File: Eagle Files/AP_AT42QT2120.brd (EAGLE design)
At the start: 36 x 45.6 mm, 20 parts

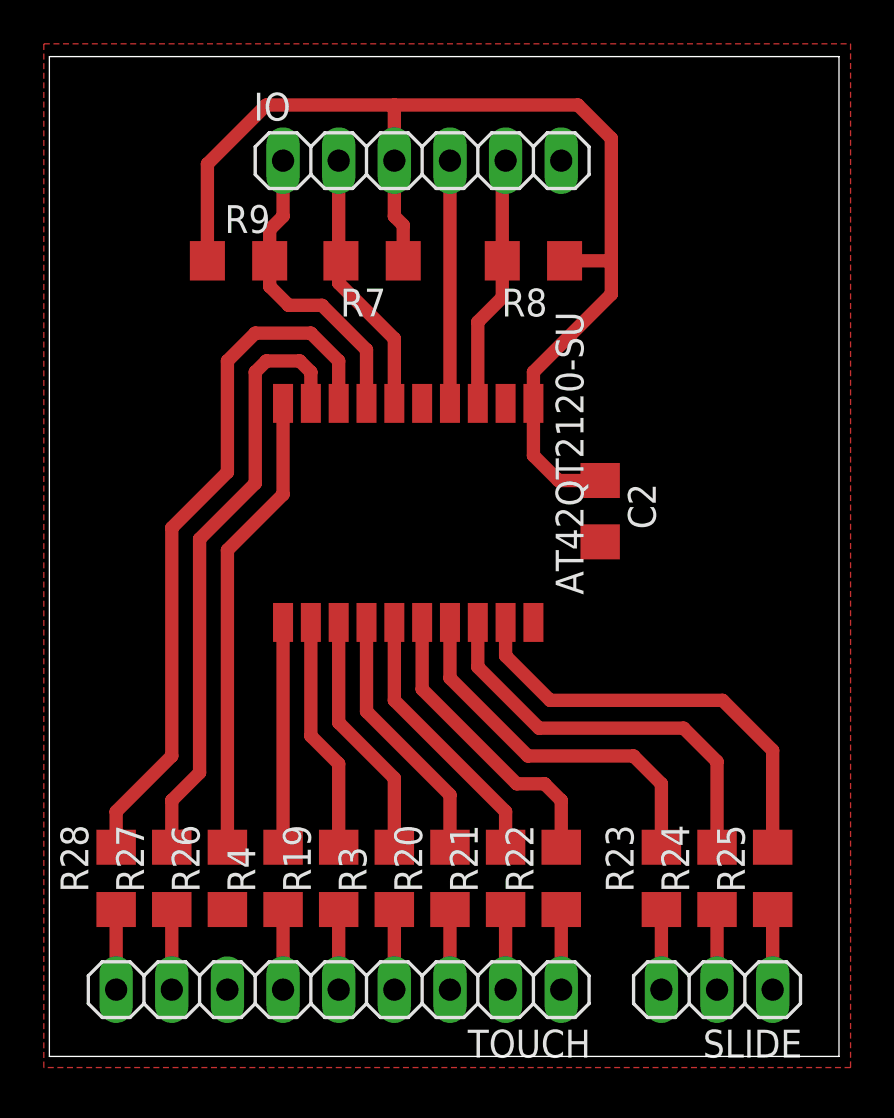
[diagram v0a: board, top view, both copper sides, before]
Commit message: pcb changes
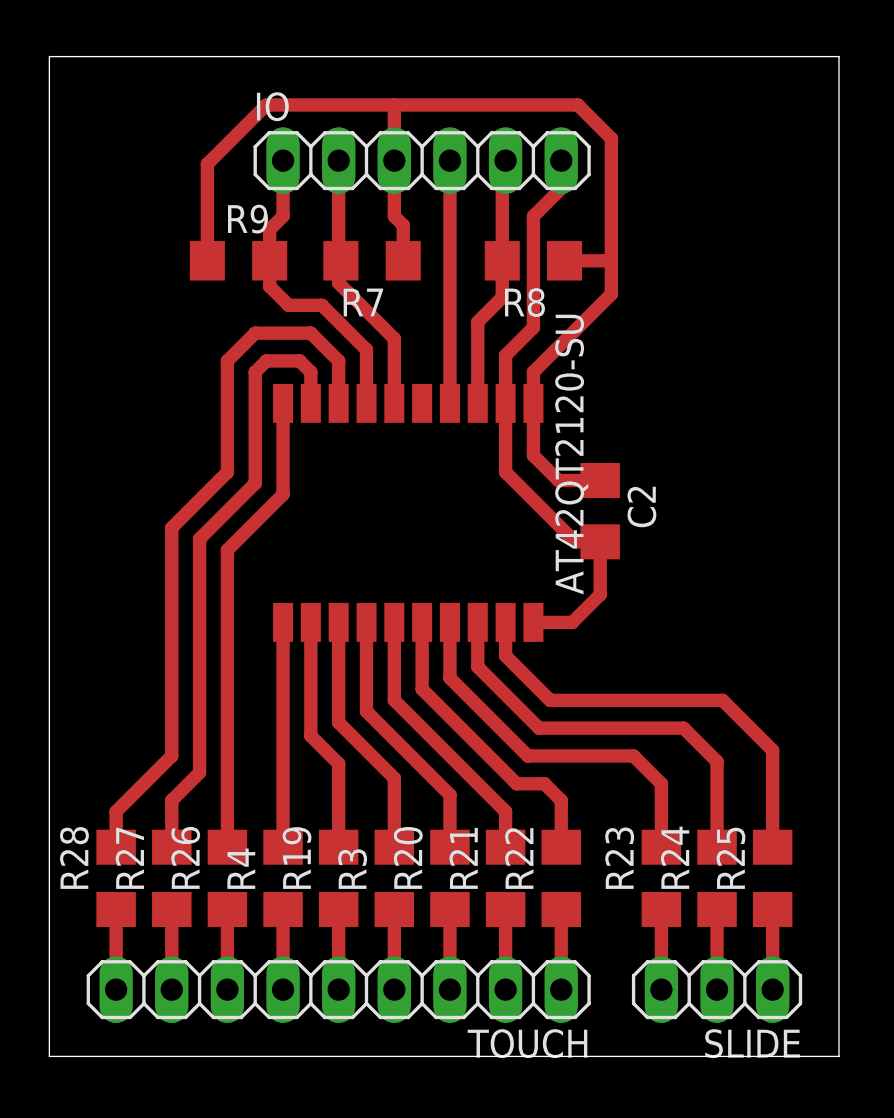
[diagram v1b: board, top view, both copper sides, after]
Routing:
- net GND: track 0.00 -> 26.9 mm
- net N$19: track 0.00 -> 3.66 mm
- removed copper zone on layer 1, net GND
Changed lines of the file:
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@@
 <contactref element="C2" pad="2"/>
 <contactref element="IO" pad="6"/>
-<polygon width="0.3048" layer="1">
-<vertex x="-0.254" y="-0.508"/>
-<vertex x="-0.254" y="46.228"/>
-<vertex x="36.576" y="46.228"/>
-<vertex x="36.576" y="-0.508"/>
-</polygon>
 <contactref element="U$1" pad="12"/>
 <contactref element="U$1" pad="10"/>
+<wire x1="23.368" y1="40.894" x2="23.368" y2="39.624" width="0.6096" layer="1"/>
+<wire x1="23.368" y1="39.624" x2="22.098" y2="38.354" width="0.6096" layer="1"/>
+<wire x1="22.098" y1="38.354" x2="22.098" y2="33.274" width="0.6096" layer="1"/>
+<wire x1="22.098" y1="33.274" x2="20.828" y2="32.004" width="0.6096" layer="1"/>
+<wire x1="20.828" y1="32.004" x2="20.828" y2="29.812" width="0.6096" layer="1"/>
+<wire x1="20.828" y1="29.812" x2="20.828" y2="26.67" width="0.6096" layer="1"/>
+<wire x1="24.006" y1="23.492" x2="25.146" y2="23.492" width="0.6096" layer="1"/>
+<wire x1="20.828" y1="26.67" x2="24.006" y2="23.492" width="0.6096" layer="1"/>
+<wire x1="22.098" y1="19.812" x2="23.876" y2="19.812" width="0.6096" layer="1"/>
+<wire x1="23.876" y1="19.812" x2="25.146" y2="21.082" width="0.6096" layer="1"/>
+<wire x1="25.146" y1="21.082" x2="25.146" y2="23.492" width="0.6096" layer="1"/>
 </signal>
 <signal name="+3V3">
@@
 <contactref element="TOUCH" pad="7"/>
 <contactref element="R26" pad="1"/>
-<wire x1="8.128" y1="3.048" x2="8.128" y2="6.706" width="0" layer="19" extent="1-1"/>
+<wire x1="8.128" y1="3.048" x2="8.128" y2="6.706" width="0.6096" layer="1"/>
 </signal>
 <signal name="N$20">
